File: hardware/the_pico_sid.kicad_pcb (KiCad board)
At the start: 4 copper layers, 18.8 x 38.6 mm, 40 parts, among them J1 Conn_01x06, Q1 2N7002, Q2 2N7002, U1 SID_6581, U2 RP2040, U3 W25Q16JVS, U4 AMS1117-3.3, U5 LM324, U6 4050, U7 4050, U8 74HC245, Y1 12MHz

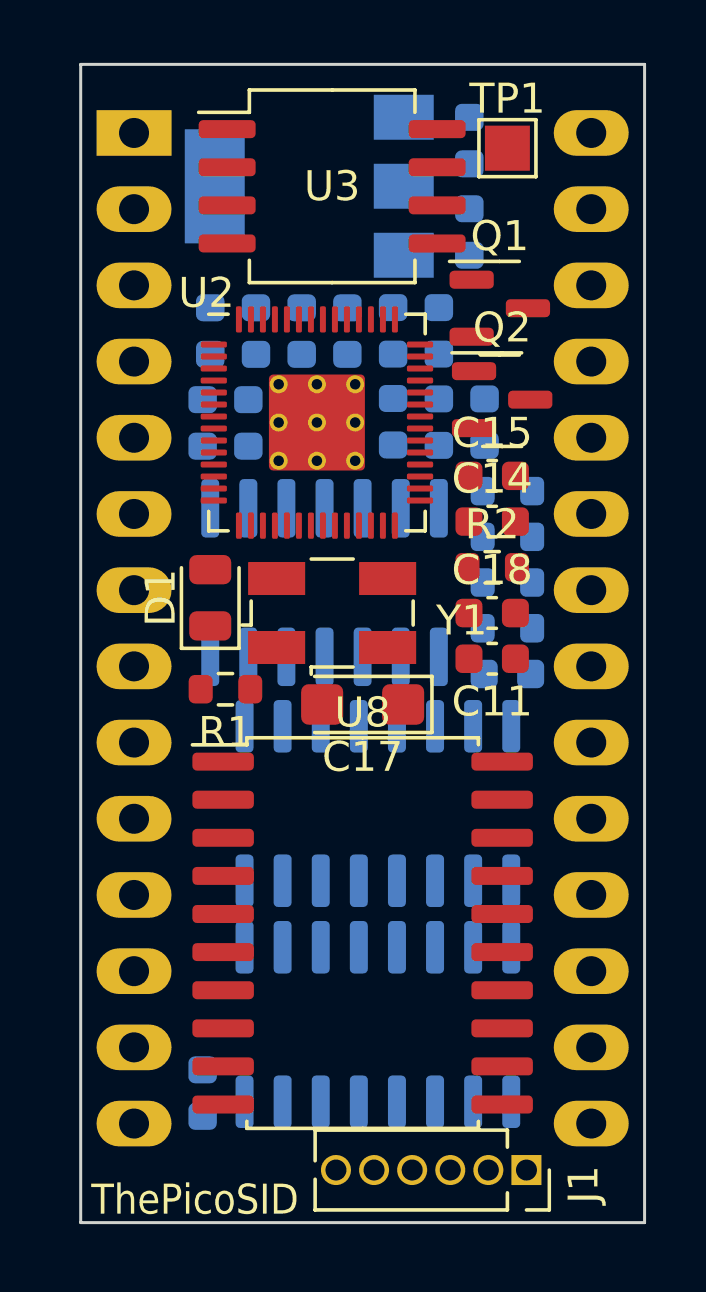
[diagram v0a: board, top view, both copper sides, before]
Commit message: convert to kicad 8.0
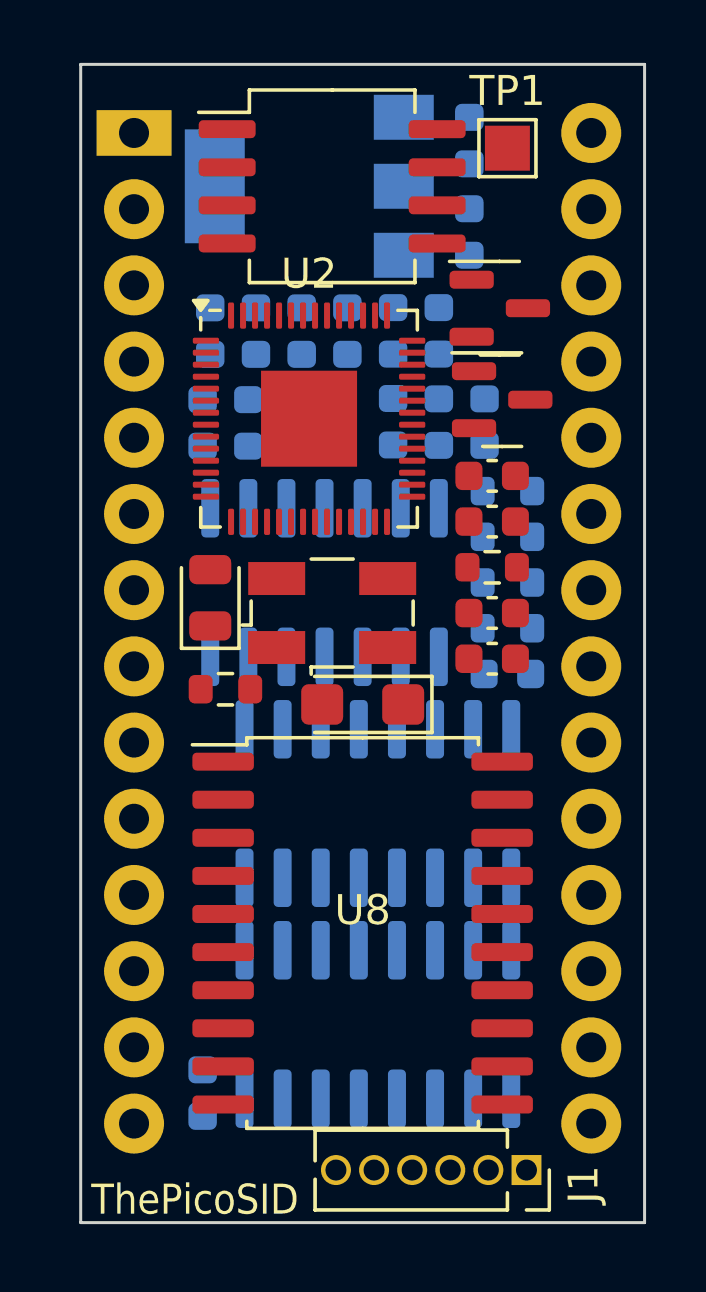
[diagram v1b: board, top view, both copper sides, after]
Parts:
- U2: footprint MCU_RaspberryPi_and_Boards:RP2040-QFN-56 -> Package_DFN_QFN:QFN-56-1EP_7x7mm_P0.4mm_EP3.2x3.2mm
- U6, U7: footprint Package_SO:SO-16_3.9x9.9mm_P1.27mm -> Package_SO:SOIC-16_3.9x9.9mm_P1.27mm
- moved U2 0.29 mm to (145.8, 90.0)
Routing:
- added copper zone on B.Cu, net GND
- added copper zone on F.Cu, net GND
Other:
- board text added: "by thorsten kattanek"

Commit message: schematic + pcb update
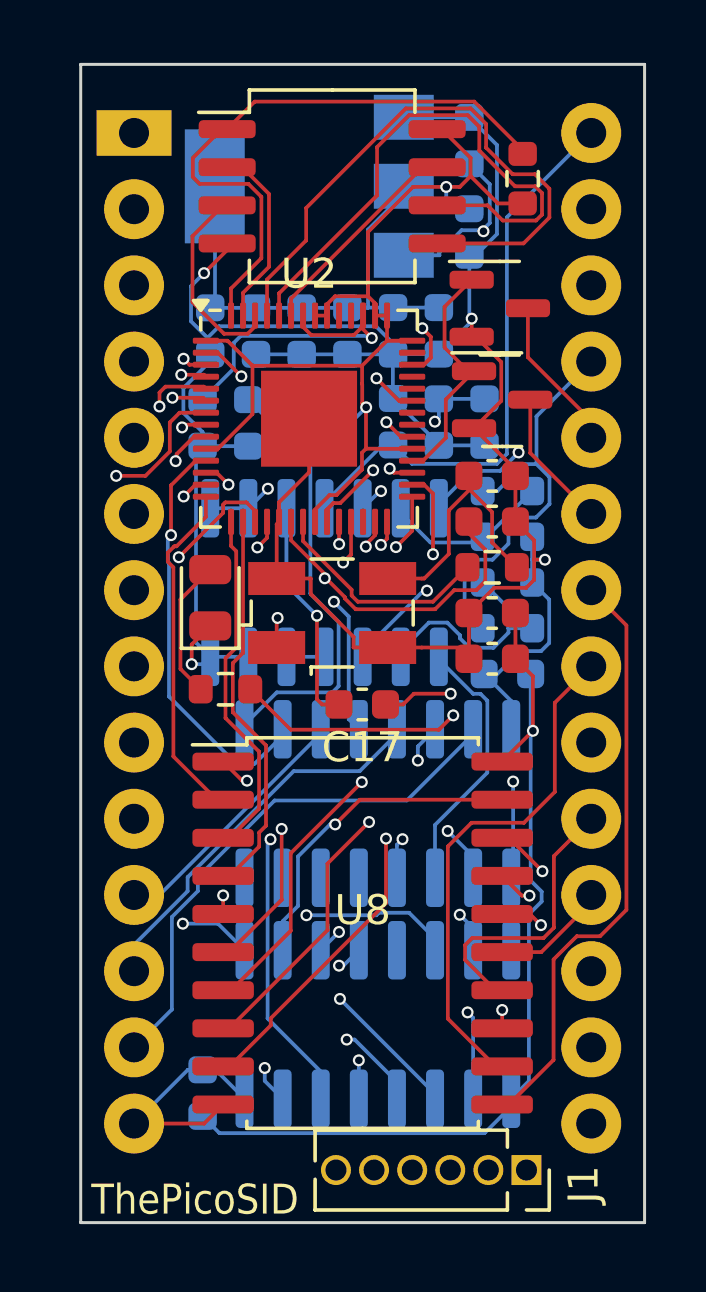
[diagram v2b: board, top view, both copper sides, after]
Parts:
- removed TP1: QSPI_SS, TestPoint:TestPoint_Pad_1.5x1.5mm
- added R2: 10k, Resistor_SMD:R_0603_1608Metric, F.Cu at (152.9, 82.0)
- C17: footprint Capacitor_Tantalum_SMD:CP_EIA-3216-18_Kemet-A -> Capacitor_SMD:C_0603_1608Metric
- renumbered C12 to C11, C13 to C12, C11 to C13, R2 to R3, R3 to R4, R4 to R5, R5 to R6, R6 to R7, U4 to U3, U3 to U4
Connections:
- C13 pad 1: Net-(U3-VCC) -> +3.3V
- J1 pad 1: GPIO22 -> GPIO00
- J1 pad 2: GPIO26 -> GPIO01
- J1 pad 3: GPIO27 -> GPIO22
- U2 pad 2: unconnected-(U2-GPIO0-Pad2) -> GPIO00
- U2 pad 3: unconnected-(U2-GPIO1-Pad3) -> GPIO01
- U2 pad 38: GPIO26 -> unconnected-(U2-GPIO26_ADC0-Pad38)
- U2 pad 39: GPIO27 -> unconnected-(U2-GPIO27_ADC1-Pad39)
- U4 pad 8: Net-(U3-VCC) -> +3.3V
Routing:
- net GND: track 0.00 -> 122.5 mm, vias 0 -> 4
- net +3.3V: track 0.00 -> 114.7 mm, vias 0 -> 3
- net GPIO01: track 0.00 -> 32.1 mm, vias 0 -> 1
- net GPIO00: track 0.00 -> 31.9 mm, vias 0 -> 1
- net RW: track 0.00 -> 30.1 mm, vias 0 -> 3
- net RES: track 0.00 -> 29.1 mm, vias 0 -> 2
- net CLK: track 0.00 -> 28.8 mm, vias 0 -> 2
- net CS: track 0.00 -> 28.6 mm, vias 0 -> 2
- net GPIO22: track 0.00 -> 26.9 mm, vias 0 -> 1
- net RES_C64: track 0.00 -> 26.2 mm, vias 0 -> 1
- net +5V: track 0.00 -> 25.5 mm, vias 0 -> 1
- net SWCLK: track 0.00 -> 22.8 mm, vias 0 -> 1
- net +1V1: track 0.00 -> 22.6 mm, vias 0 -> 3
- net CLK_C64: track 0.00 -> 22.6 mm, vias 0 -> 1
- net SWD: track 0.00 -> 22.3 mm, vias 0 -> 1
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- removed copper zone on B.Cu, net GND
- removed copper zone on F.Cu, net GND
